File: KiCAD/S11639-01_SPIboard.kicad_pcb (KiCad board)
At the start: 4 copper layers, 70 x 40 mm, 60 parts, among them IC1 74LVC1T45GW,125, IC2 74LVC1T45GW,125, IC3 74LVC1T45GW,125, IC4 MCP33131D-10-I_MS, IC5 74LVC1T45GW,125, J1 Conn_01x03_Male, J2 Conn_02x10_Odd_Even, J3 705430001, J4 Conn_01x03_Male, U1 ADA4807-2ARMZ-R7, U2 LT1761-BYP, U3 TPS72218

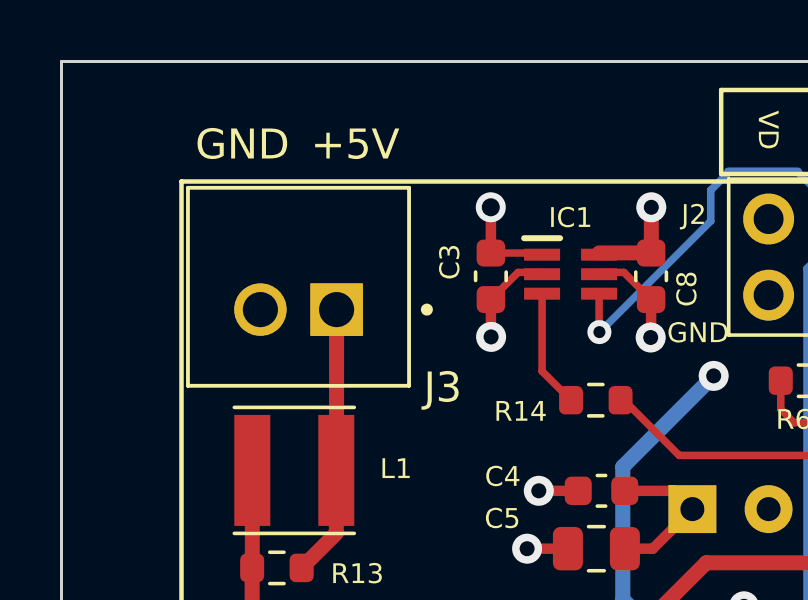
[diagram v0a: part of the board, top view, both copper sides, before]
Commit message: Add files via upload
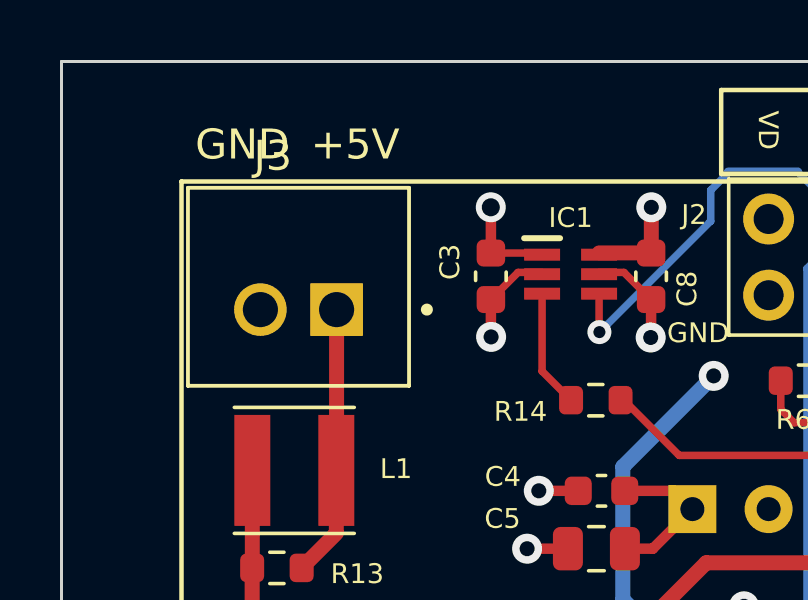
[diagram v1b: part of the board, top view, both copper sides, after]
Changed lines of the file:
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@@
     (descr "Capacitor SMD 0603 (1608 Metric), square (rectangular) end terminal, IPC_7351 nominal, (Body size source: IPC-SM-782 page 76, https://www.pcb-3d.com/wordpress/wp-content/uploads/ipc-sm-782a_amendment_1_and_2.pdf), generated with kicad-footprint-generator")
     (tags "capacitor")
-    (property "Description" "CAP CER 1000PF 25V C0G/NP0 0603")
-    (property "Digikey" "399-C0603C102F3GAC7867CT-ND")
+    (property "Description" "CAP CER 1000PF 50V C0G/NPO 0603")
+    (property "Digikey" "311-1743-1-ND")
     (property "Sheetfile" "S11639-01_SPIboard.kicad_sch")
     (property "Sheetname" "")
@@
     (descr "Capacitor SMD 0603 (1608 Metric), square (rectangular) end terminal, IPC_7351 nominal, (Body size source: IPC-SM-782 page 76, https://www.pcb-3d.com/wordpress/wp-content/uploads/ipc-sm-782a_amendment_1_and_2.pdf), generated with kicad-footprint-generator")
     (tags "capacitor")
-    (property "Description" "CAP CER 1000PF 25V C0G/NP0 0603")
-    (property "Digikey" "399-C0603C102F3GAC7867CT-ND")
+    (property "Description" "CAP CER 1000PF 50V C0G/NPO 0603")
+    (property "Digikey" "311-1743-1-ND")
     (property "Sheetfile" "S11639-01_SPIboard.kicad_sch")
     (property "Sheetname" "")
@@
     (property "Sheetname" "")
     (attr through_hole)
-    (fp_text reference "J3" (at 4.81 2.6) (layer "F.SilkS")
+    (fp_text reference "J3" (at -0.855 -5.125) (layer "F.SilkS")
       (effects (font (size 1 1) (thickness 0.15)))
     )
@@
       (effects (font (size 1 1) (thickness 0.15)))
     )
+    (fp_line (start 3.685 2.54) (end -3.685 2.54) (layer "F.SilkS") (width 0.127))
     (fp_line (start -3.685 2.54) (end -3.685 -4.06) (layer "F.SilkS") (width 0.127))
     (fp_line (start -3.685 -4.06) (end 3.685 -4.06) (layer "F.SilkS") (width 0.127))
-    (fp_line (start 3.685 2.54) (end -3.685 2.54) (layer "F.SilkS") (width 0.127))
     (fp_line (start 3.685 -4.06) (end 3.685 2.54) (layer "F.SilkS") (width 0.127))
     (fp_circle (center 4.28 0) (end 4.38 0) (layer "F.SilkS") (width 0.2) (fill none))
     (fp_line (start 3.935 -4.31) (end 3.935 2.79) (layer "F.CrtYd") (width 0.05))
+    (fp_line (start -3.935 -4.31) (end 3.935 -4.31) (layer "F.CrtYd") (width 0.05))
+    (fp_line (start -3.935 2.79) (end -3.935 -4.31) (layer "F.CrtYd") (width 0.05))
     (fp_line (start 3.935 2.79) (end -3.935 2.79) (layer "F.CrtYd") (width 0.05))
-    (fp_line (start -3.935 2.79) (end -3.935 -4.31) (layer "F.CrtYd") (width 0.05))
-    (fp_line (start -3.935 -4.31) (end 3.935 -4.31) (layer "F.CrtYd") (width 0.05))
     (fp_line (start 3.685 -4.06) (end 3.685 2.54) (layer "F.Fab") (width 0.127))
     (fp_line (start 3.685 2.54) (end -3.685 2.54) (layer "F.Fab") (width 0.127))
